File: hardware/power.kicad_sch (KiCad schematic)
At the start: 17 parts, among them Q2 SI2347DS-T1-GE3, U7 NCP565D2T33R4G, U8 SI06W8-05

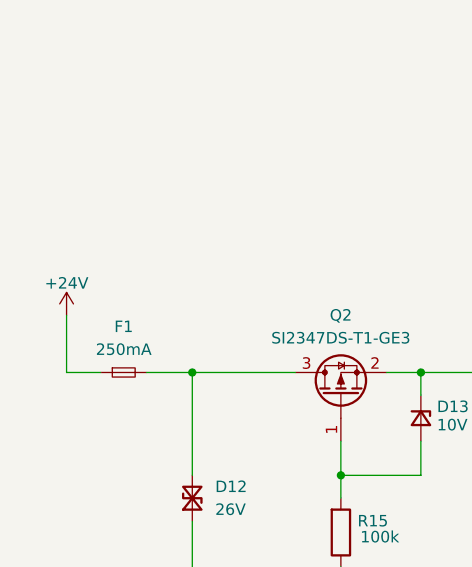
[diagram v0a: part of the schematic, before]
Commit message: mistake correction
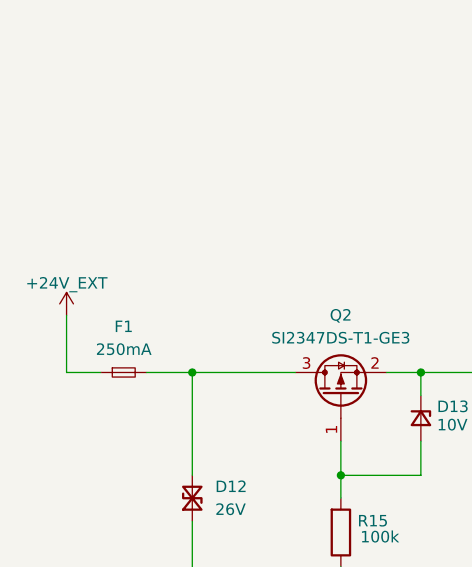
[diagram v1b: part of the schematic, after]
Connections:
- net +24V renamed +24V_EXT
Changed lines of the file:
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@@
 			)
 		)
-		(property "Value" "+24V"
+		(property "Value" "+24V_EXT"
 			(at 52.07 72.644 0)
 			(show_name no)
